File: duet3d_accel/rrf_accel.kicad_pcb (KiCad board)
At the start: 2 copper layers, 100 x 100 mm, 13 parts, among them J1 Conn_02x05_Odd_Even, U1 LIS3DH

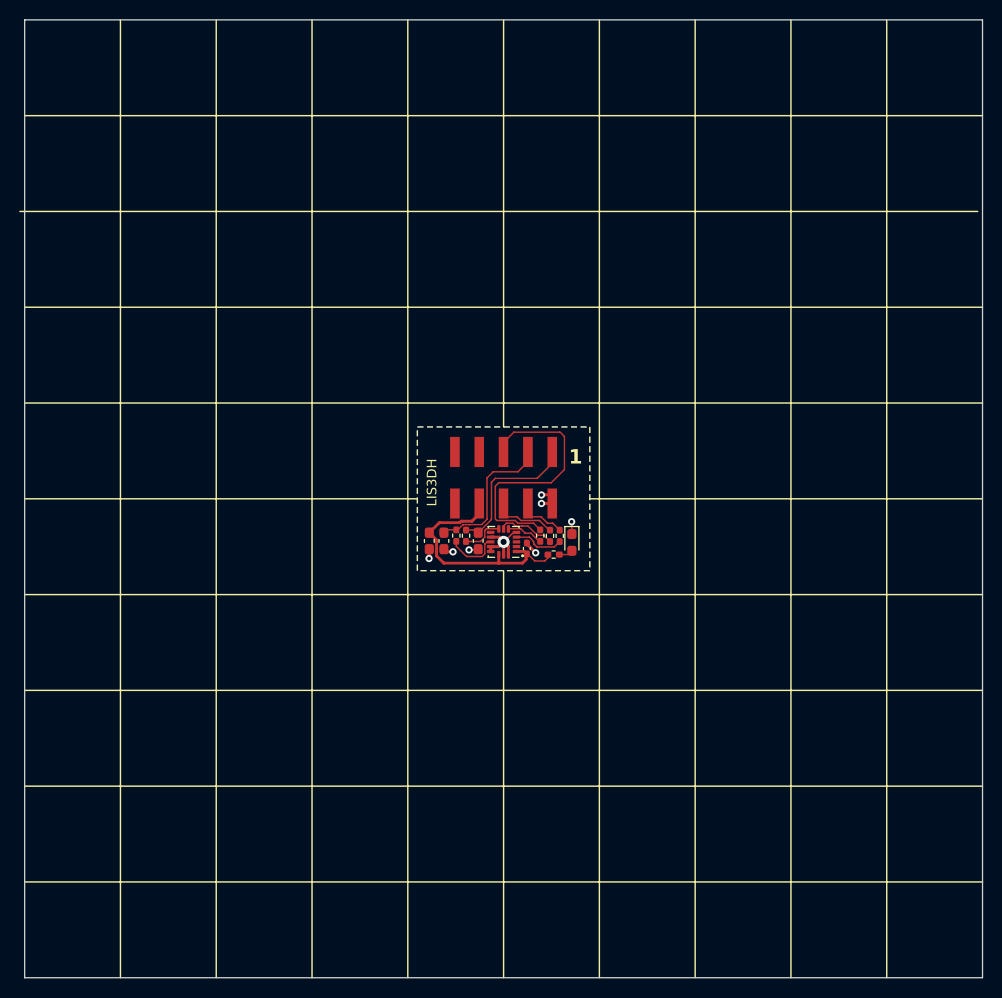
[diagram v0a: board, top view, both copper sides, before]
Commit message: Tweaked the layout
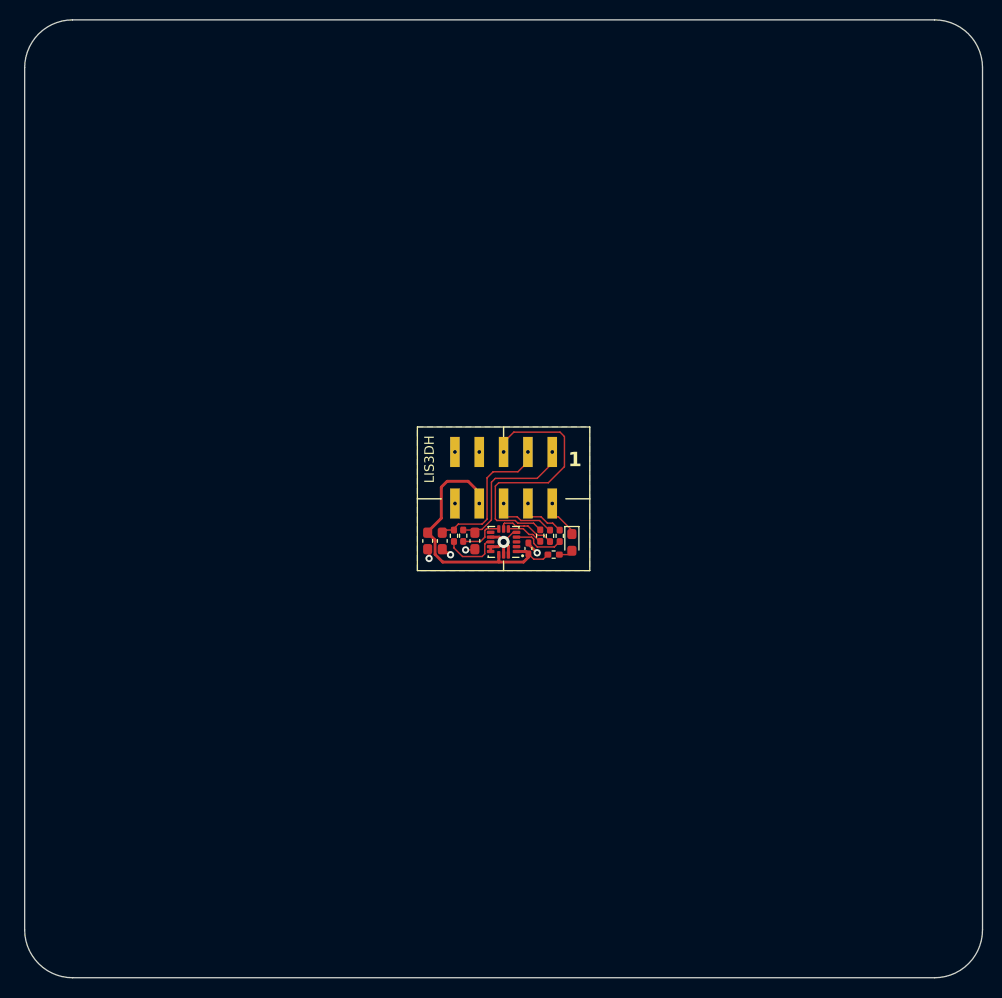
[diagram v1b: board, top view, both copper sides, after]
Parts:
- moved C4 0.35 mm to (-3.00, 4.40)
- moved R6 0.30 mm to (-4.22, 3.86)
- moved R1 0.25 mm to (-5.18, 3.86)
- moved C1 0.17 mm to (-7.92, 4.40)
- moved C3 0.17 mm to (-6.40, 4.40)
- moved C2 0.16 mm to (2.59, 5.18)
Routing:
- net +3V3: track 25.3 -> 28.8 mm
- net /CS: track 15.8 -> 14.7 mm
- net GNDD: track 15.8 -> 14.9 mm, vias 8 -> 5
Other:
- outline, holes or cut-outs redrawn
